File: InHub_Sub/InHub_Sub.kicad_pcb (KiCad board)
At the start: 2 copper layers, 20 parts, among them J1 Conn_01x02, SW1 SW_Push, U1 AMS1117-3.3, U2 STM32L011F4Px, U3 NRF24L01_Breakout, Y1 32.768kHz

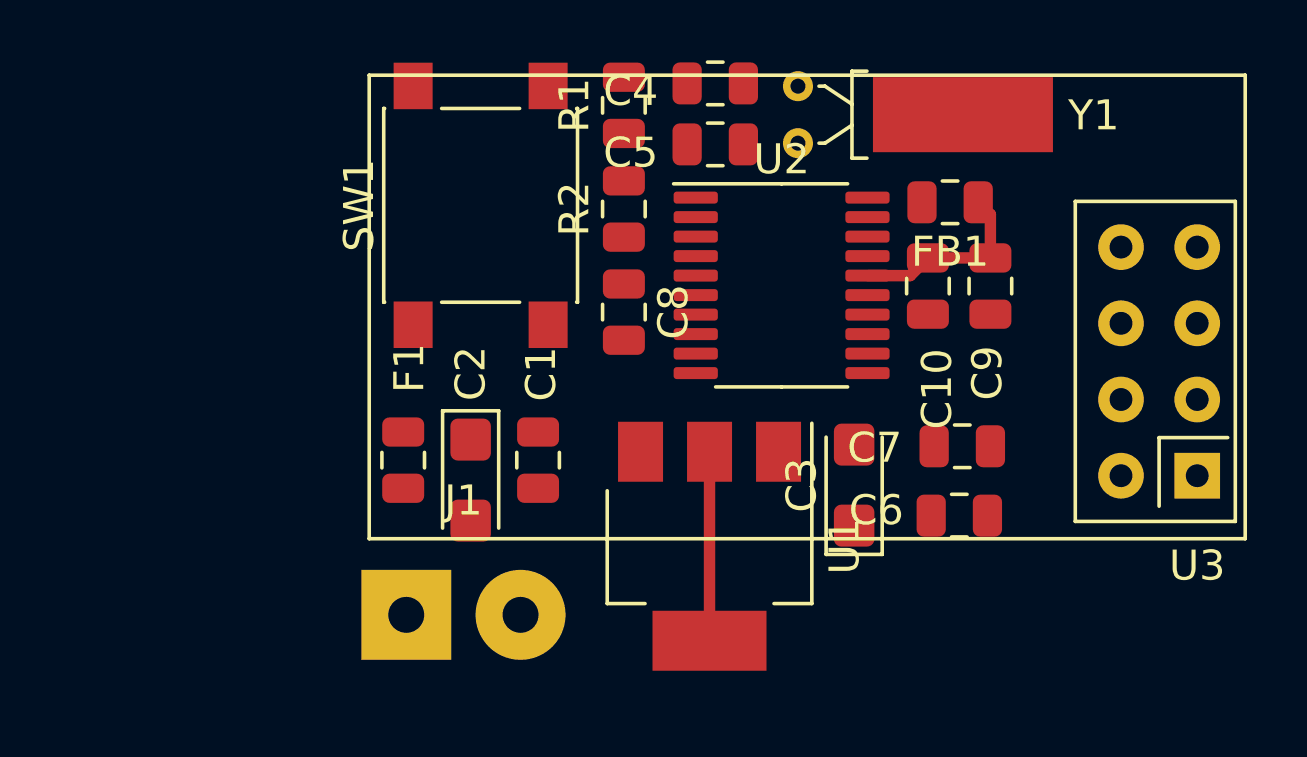
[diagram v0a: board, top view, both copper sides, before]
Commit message: change
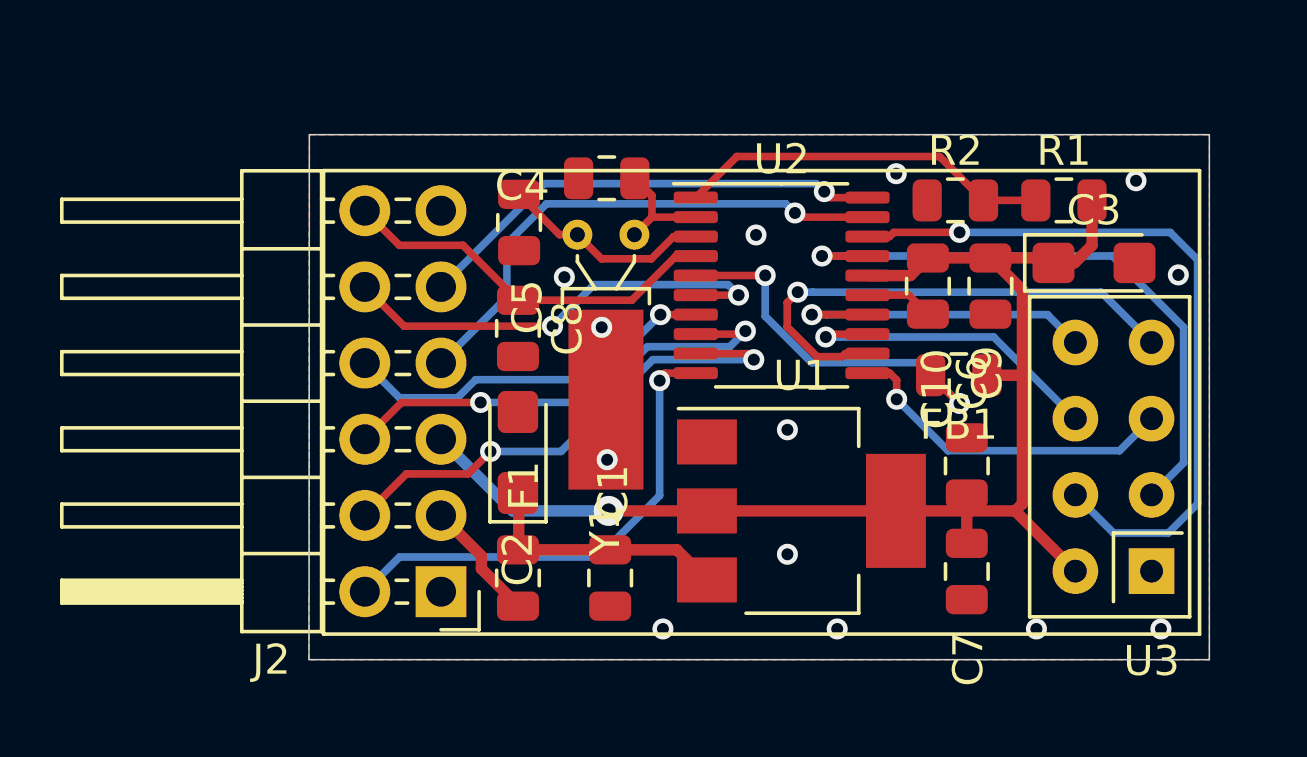
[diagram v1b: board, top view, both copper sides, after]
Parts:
- removed J1: Conn_01x02, Connector_Wire:SolderWirePad_1x02_P3.81mm_Drill1.2mm
- removed SW1: SW_Push, Button_Switch_SMD:SW_SPST_PTS645
- added J2: Conn_02x06_Odd_Even, Connector_PinHeader_2.54mm:PinHeader_2x06_P2.54mm_Horizontal, F.Cu at (52.6, 89.7)
- moved R1 15.0 mm to (73.3, 76.6), turned to 0 degrees
- moved R2 11.1 mm to (69.7, 76.6), turned to 0 degrees
- moved C3 10.9 mm to (74.3, 78.7), turned to 0 degrees
- moved Y1 7.96 mm to (57.1, 77.8), turned to 0 degrees
- moved C5 7.04 mm to (55.2, 77.4), turned to 270 degrees
- moved FB1 5.77 mm to (69.8, 82.4)
- moved F1 5.48 mm to (55.1, 89.2)
- moved C4 4.80 mm to (58.1, 75.9)
- moved C1 4.60 mm to (58.2, 89.2)
- moved C7 4.18 mm to (70.1, 89.0), turned to 270 degrees
- moved C8 3.57 mm to (55.1, 80.9)
- moved U3 3.53 mm to (76.3, 89.0)
- moved U1 3.28 mm to (64.6, 87.0), turned to 0 degrees
- moved C2 1.83 mm to (55.1, 85.0), turned to 90 degrees
- moved C6 1.67 mm to (70.1, 85.5), turned to 90 degrees
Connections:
- net Net-(C8-Pad1) renamed /NRST
- U2 pad 10: Net-(U2-Pad10) -> /PA4
- U2 pad 6: Net-(U2-Pad6) -> /PA0
- U2 pad 7: Net-(U2-Pad7) -> /PA1
- U2 pad 8: Net-(U2-Pad8) -> /PA2
- U2 pad 9: Net-(U2-Pad9) -> /PA3
- Y1 pad 3: (no net) -> GND
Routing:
- net +3V3: track 12.7 -> 44.3 mm, vias 0 -> 1
- net /nRF24L01_CSN: track 0.00 -> 24.6 mm, vias 0 -> 1
- net /nRF24L01_CE: track 0.00 -> 20.6 mm, vias 0 -> 1
- net /SWDIO: track 0.00 -> 17.6 mm, vias 0 -> 1
- net /PA3: track 0.00 -> 17.1 mm, vias 0 -> 2
- net /nRF24L01_MISO: track 0.00 -> 16.9 mm, vias 0 -> 1
- net /PA4: track 0.00 -> 16.3 mm, vias 0 -> 1
- net /PA2: track 0.00 -> 15.9 mm, vias 0 -> 2
- net /SWCLK: track 0.00 -> 15.8 mm, vias 0 -> 1
- net /PA0: track 0.00 -> 15.1 mm, vias 0 -> 2
- net /NRST: track 0.00 -> 12.9 mm
- net +3.3VA: track 0.00 -> 12.7 mm, vias 0 -> 2
- net /PA1: track 0.00 -> 12.7 mm, vias 0 -> 1
- net /BOOT0: track 0.00 -> 12.5 mm
- net /nRF24L01_SCK: track 0.00 -> 11.4 mm, vias 0 -> 1
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- added copper zone on B.Cu, net GND
- added copper zone on F.Cu, net GND
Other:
- board outline added: 30 x 17.5 mm
- net class Default: via_dia 0.8 -> 0.7
